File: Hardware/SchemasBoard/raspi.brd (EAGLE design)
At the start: 14.1 x 25.3 mm, 7 parts

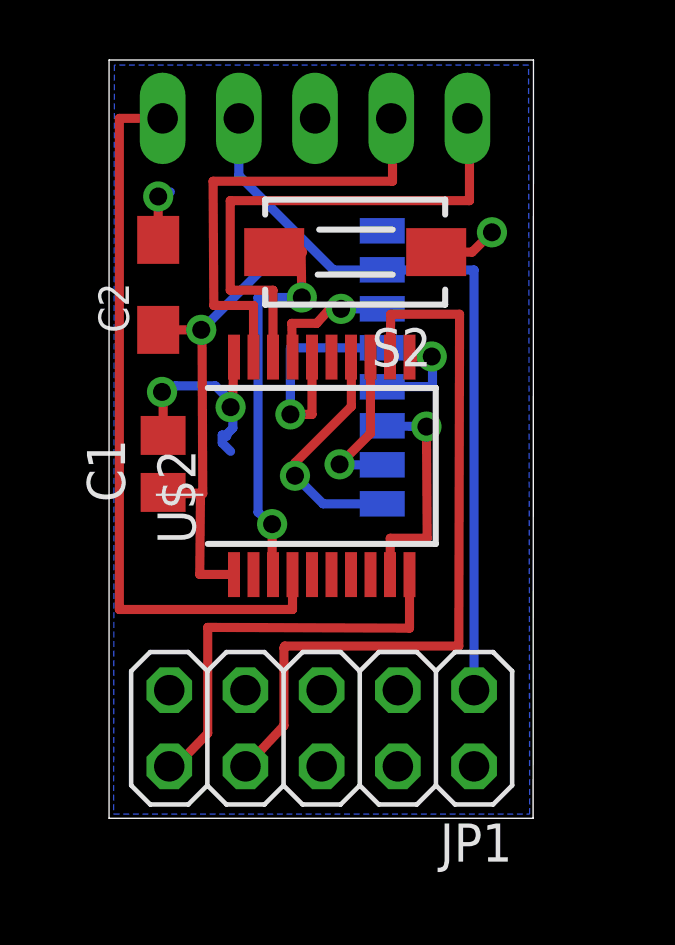
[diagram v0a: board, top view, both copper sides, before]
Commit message: aa
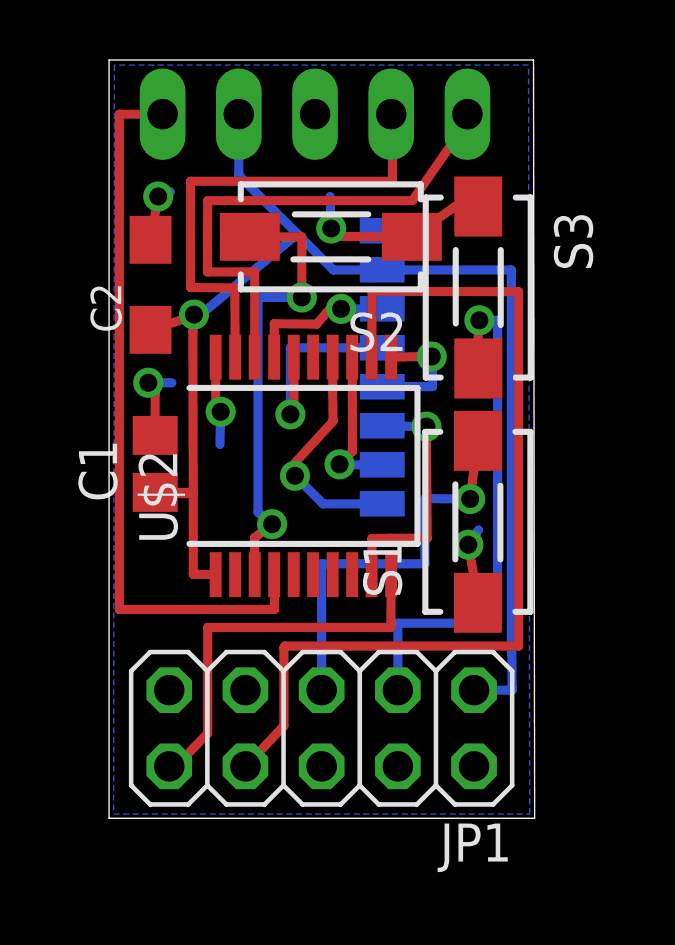
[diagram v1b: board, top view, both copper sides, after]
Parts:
- added S1, S3: DTSM-3, switch-tact:DTSM-3
- moved S2 0.96 mm to (7.39, 19.4)
- moved U$2 0.61 mm to (6.48, 11.7)
- moved C1 0.27 mm to (1.54, 11.8)
- moved C2 0.25 mm to (1.38, 17.8)
- moved JP2 0.14 mm to (6.87, 23.5)
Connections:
- new net N$1: JP1.3, S3.2
- new net N$2: JP1.5, S1.2
- net GND: now also S1.1, S3.1
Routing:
- net N$1: track 0.00 -> 17.9 mm, vias 0 -> 1
- net N$2: track 0.00 -> 13.3 mm, vias 0 -> 1
- net N$34: track 25.1 -> 31.2 mm
- net GND: track 12.5 -> 16.5 mm, vias 4 -> 5
- net VDD: track 43.0 -> 45.7 mm
- net N$28: track 13.7 -> 15.3 mm
- net N$18: track 15.3 -> 16.3 mm
- net N$33: track 13.8 -> 13.1 mm
- net N$20: track 7.91 -> 7.29 mm
- net N$22: track 3.48 -> 4.09 mm
- net N$23: track 7.65 -> 8.24 mm
- net N$16: track 4.37 -> 4.96 mm
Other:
- board size 14.1 x 25.3 mm -> 14.2 x 25.3 mm

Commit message: a
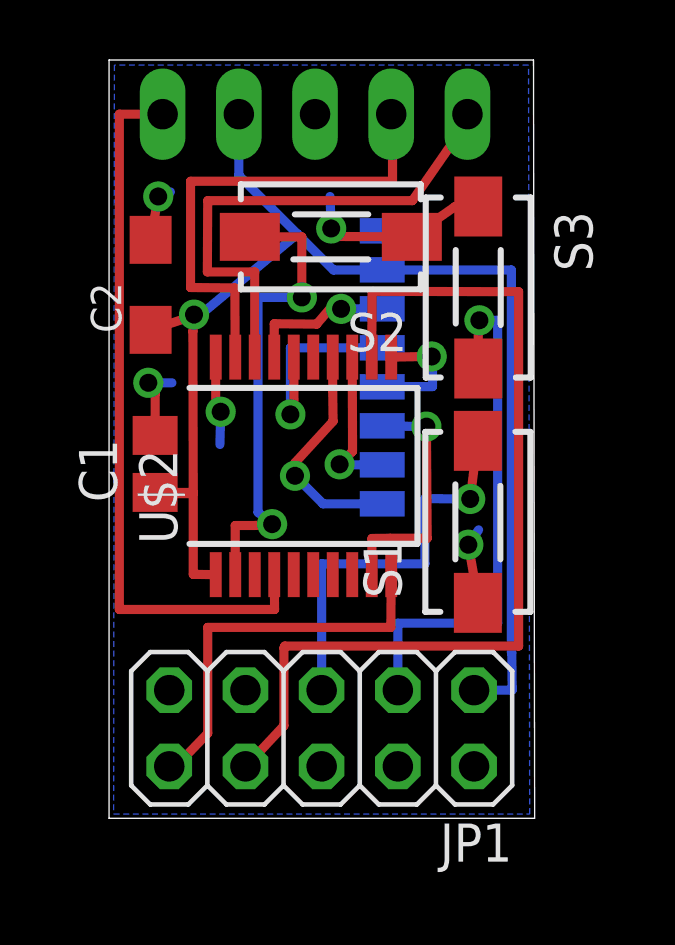
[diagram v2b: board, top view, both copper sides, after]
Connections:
- net N$28: now also U$2.2; no longer U$2.3
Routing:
- net N$28: track 15.3 -> 16.2 mm
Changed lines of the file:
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@@
 </signal>
 <signal name="N$28">
-<contactref element="U$2" pad="3"/>
 <contactref element="S2" pad="2"/>
 <wire x1="4.6914" y1="19.3802" x2="6.4262" y2="19.3802" width="0.3048" layer="1"/>
@@
 <wire x1="6.4262" y1="17.3609" x2="4.9657" y2="17.3609" width="0.3048" layer="16"/>
 <wire x1="4.9657" y1="17.3609" x2="4.9657" y2="10.1981" width="0.3048" layer="16"/>
-<wire x1="4.8553" y1="8.1211" x2="4.8514" y2="9.353" width="0.3048" layer="1"/>
-<wire x1="4.8514" y1="9.353" x2="5.4356" y2="9.8044" width="0.3048" layer="1"/>
+<wire x1="4.8514" y1="9.7594" x2="5.4356" y2="9.8044" width="0.3048" layer="1"/>
 <via x="5.4356" y="9.8044" extent="1-16" drill="0.6"/>
 <wire x1="5.4356" y1="9.8044" x2="4.9657" y2="10.1981" width="0.3048" layer="16"/>
+<contactref element="U$2" pad="2"/>
+<wire x1="4.8514" y1="9.7594" x2="4.2053" y2="9.7594" width="0.3048" layer="1"/>
+<wire x1="4.2053" y1="9.7594" x2="4.2053" y2="8.1211" width="0.3048" layer="1"/>
 </signal>
 <signal name="N$33">
